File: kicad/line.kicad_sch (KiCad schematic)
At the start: 40 parts, among them J11 AudioJack3, J2 AudioJack3, U12 NE5532, U13 NE5532, U14 NE5532, U15 NE5532

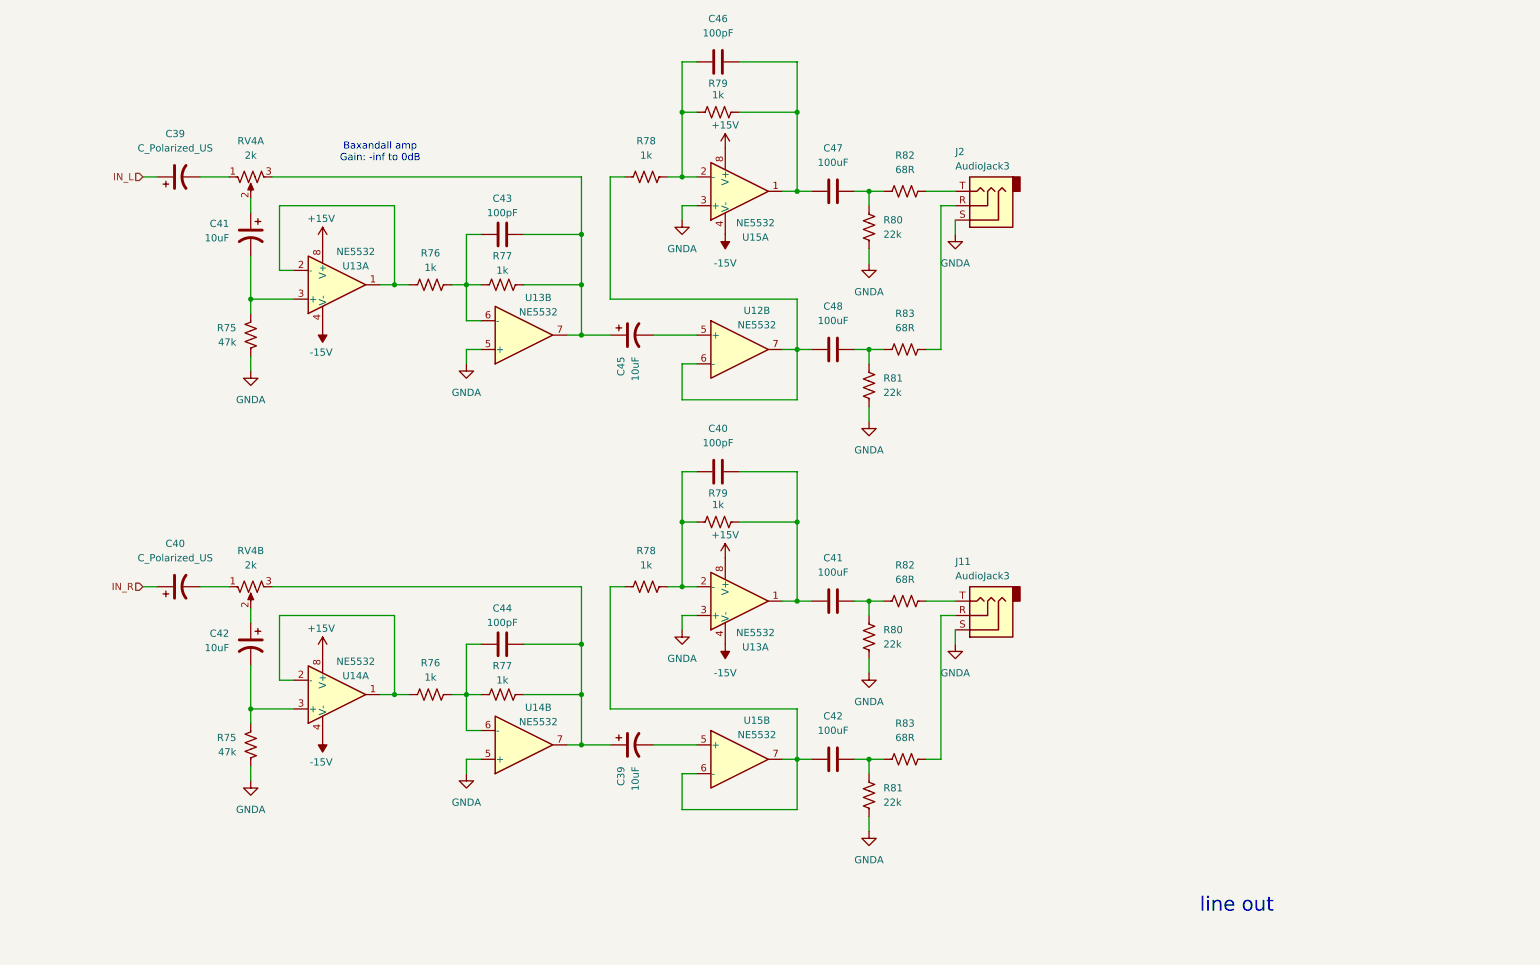
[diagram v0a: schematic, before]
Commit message: tac5212 initial architecture
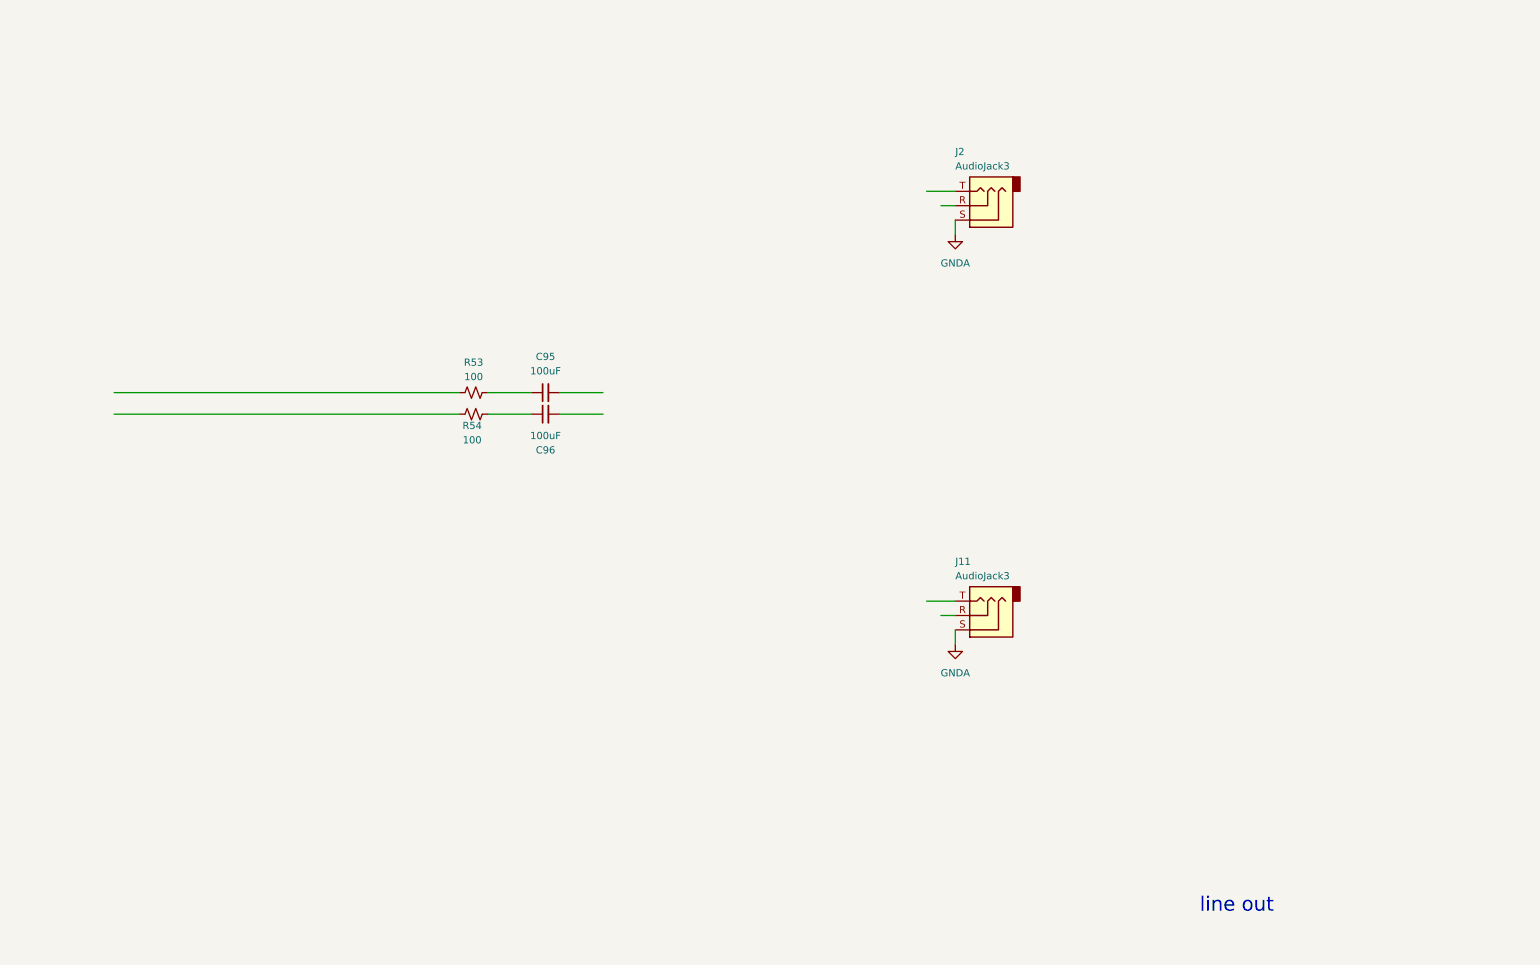
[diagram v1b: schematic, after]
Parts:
- removed C39, C40: C_Polarized_US, symbol Device:C_Polarized_US
- removed C39, C41, C42, C45: 10uF, symbol Device:C_Polarized_US
- removed C40, C43, C44, C46: 100pF, symbol Device:C
- removed C41, C42, C47, C48: 100uF, symbol Device:C
- removed R75 (x2): 47k, symbol Device:R_US
- removed R76 (x2), R77 (x2), R78 (x2), R79 (x2): 1k, symbol Device:R_US
- removed R80 (x2), R81 (x2): 22k, symbol Device:R_US
- removed R82 (x2), R83 (x2): 68R, symbol Device:R_US
- removed RV4: 2k, symbol openmic:R_Potentiometer_US_Dual
- removed U12, U13, U14, U15: NE5532, symbol Amplifier_Operational:NE5532
- added C95, C96: 100uF, symbol Device:C_Small
- added R53, R54: 100, symbol Device:R_Small_US
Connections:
- new net: C95.1, R53.2
- new net: C96.1, R54.2
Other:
- note removed: "Baxandall amp Gain: -inf to 0dB"

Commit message: line out
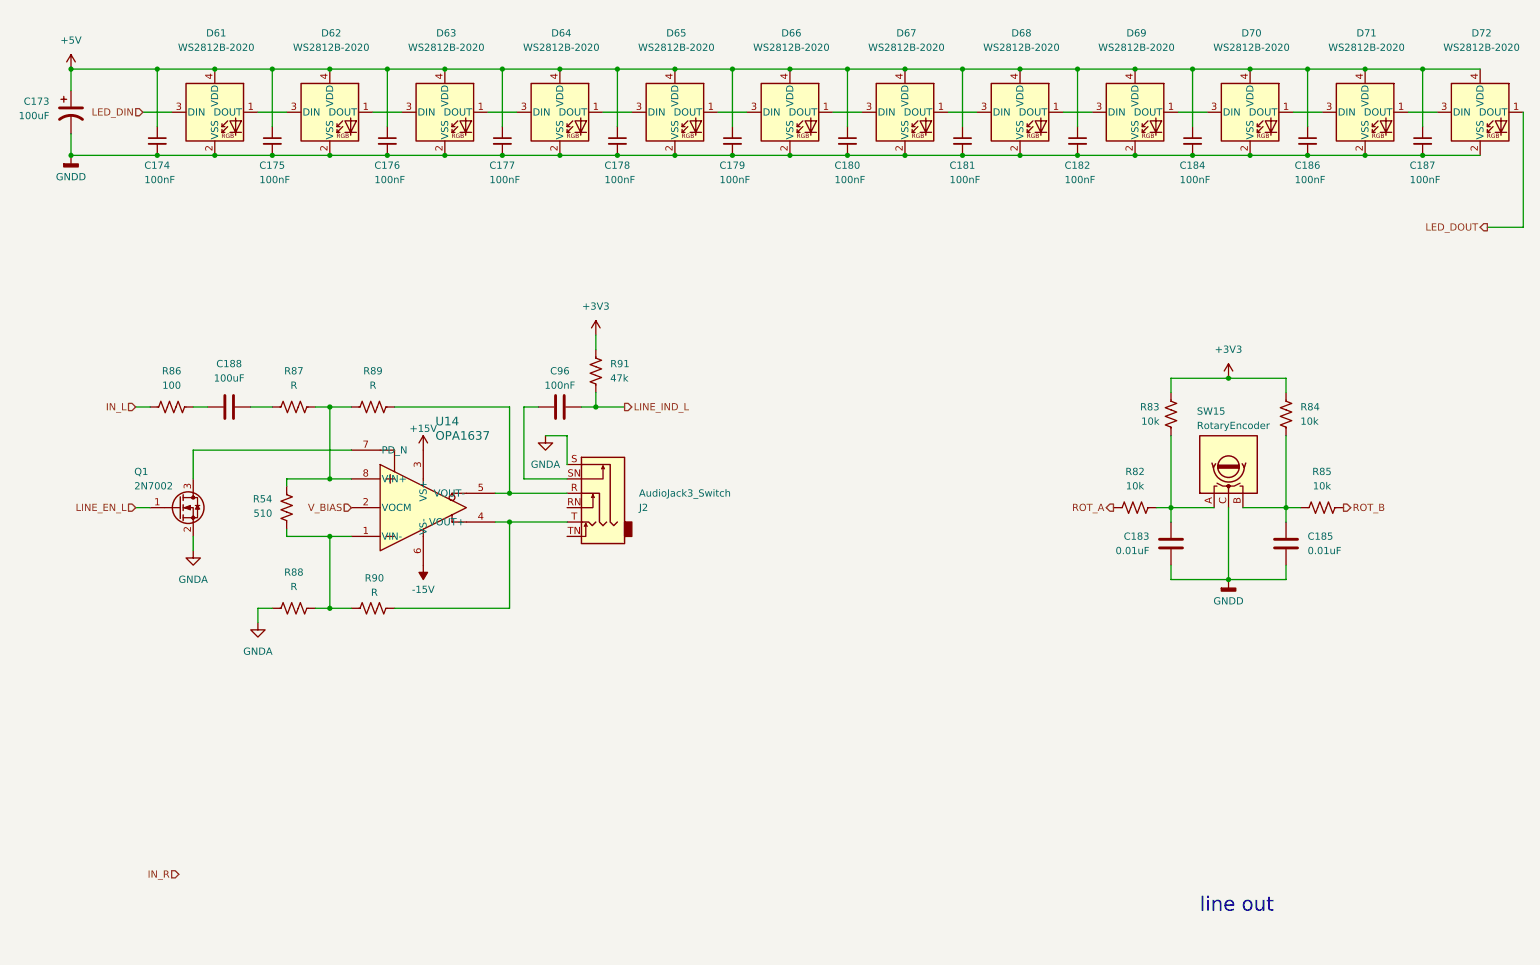
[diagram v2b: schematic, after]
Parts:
- removed C95, C96: 100uF, symbol Device:C_Small
- removed J11, J2: AudioJack3, symbol Connector_Audio:AudioJack3
- removed R53, R54: 100, symbol Device:R_Small_US
- added C173: 100uF, symbol Device:C_Polarized_US
- added C174, C175, C176, C177, C178, C179, C180, C181, C182, C184, C186, C187: 100nF, symbol Device:C_Small
- added C183, C185: 0.01uF, symbol Device:C
- added C188: 100uF, symbol Device:C
- added C96: 100nF, symbol Device:C
- added D61, D62, D63, D64, D65, D66, D67, D68, D69, D70, D71, D72: WS2812B-2020, LED_SMD:LED_WS2812B-2020_PLCC4_2.0x2.0mm, symbol LED:WS2812B-2020
- added J2: AudioJack3_Switch, symbol Connector_Audio:AudioJack3_Switch
- added Q1: 2N7002, Package_TO_SOT_SMD:SOT-23, symbol Transistor_FET:2N7002
- added R54: 510, symbol Device:R_US
- added R82, R83, R84, R85: 10k, symbol Device:R_US
- added R86: 100, symbol Device:R_US
- added R87, R88, R89, R90: R, symbol Device:R_US
- added R91: 47k, symbol Device:R_US
- added SW15: RotaryEncoder, symbol Device:RotaryEncoder
- added U14: OPA1637, DGK0008A_N, symbol openmic:OPA1637
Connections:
- net GNDA: now also J2.S, Q1.2 (S), R88.1
- new net: C96.1, J2.SN
- new net: D69.1 (DOUT), D70.3 (DIN)
- new net: D68.1 (DOUT), D69.3 (DIN)
- new net: D67.1 (DOUT), D68.3 (DIN)
- new net: D66.1 (DOUT), D67.3 (DIN)
- new net: J2.T, R90.1, U14.4 (VOUT+)
- new net: R54.1, R88.2, R90.2, U14.1 (VIN-)
- new net: D71.1 (DOUT), D72.3 (DIN)
- new net: D70.1 (DOUT), D71.3 (DIN)
- new net: C183.1, R82.2, R83.1, SW15.A
- new net: C185.1, R84.2, R85.1, SW15.B
- new net: R54.2, R87.2, R89.1, U14.8 (VIN+)
- new net: J2.R, R89.2, U14.5 (VOUT-)
- new net: D65.1 (DOUT), D66.3 (DIN)
- new net: D64.1 (DOUT), D65.3 (DIN)
- new net: Q1.3 (D), U14.7 (PD_N)
- new net: D61.1 (DOUT), D62.3 (DIN)
- new net: D63.1 (DOUT), D64.3 (DIN)
- new net: D62.1 (DOUT), D63.3 (DIN)
- new net: C188.1, R86.2
- new net: C188.2, R87.1
- new net +15V: U14.3 (VS+)
- new net +3V3: R83.2, R84.1, R91.1
- new net +5V: C173.1, C174.1, C175.1, C176.1, C177.1, C178.1, C179.1, C180.1, C181.1, C182.1, C184.1, C186.1, C187.1, D61.4 (VDD), D62.4 (VDD), D63.4 (VDD), D64.4 (VDD), D65.4 (VDD), D66.4 (VDD), D67.4 (VDD), D68.4 (VDD), D69.4 (VDD), D70.4 (VDD), D71.4 (VDD), D72.4 (VDD)
- new net -15V: U14.6 (VS-)
- new net GNDD: C173.2, C174.2, C175.2, C176.2, C177.2, C178.2, C179.2, C180.2, C181.2, C182.2, C183.2, C184.2, C185.2, C186.2, C187.2, D61.2 (VSS), D62.2 (VSS), D63.2 (VSS), D64.2 (VSS), D65.2 (VSS), D66.2 (VSS), D67.2 (VSS), D68.2 (VSS), D69.2 (VSS), D70.2 (VSS), D71.2 (VSS), D72.2 (VSS), SW15.C
- new net IN_L: R86.1
- new net LED_DIN: D61.3 (DIN)
- new net LED_DOUT: D72.1 (DOUT)
- new net LINE_EN_L: Q1.1 (G)
- new net LINE_IND_L: C96.2, R91.2
- new net ROT_A: R82.1
- new net ROT_B: R85.2
- new net V_BIAS: U14.2 (VOCM)

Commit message: line out
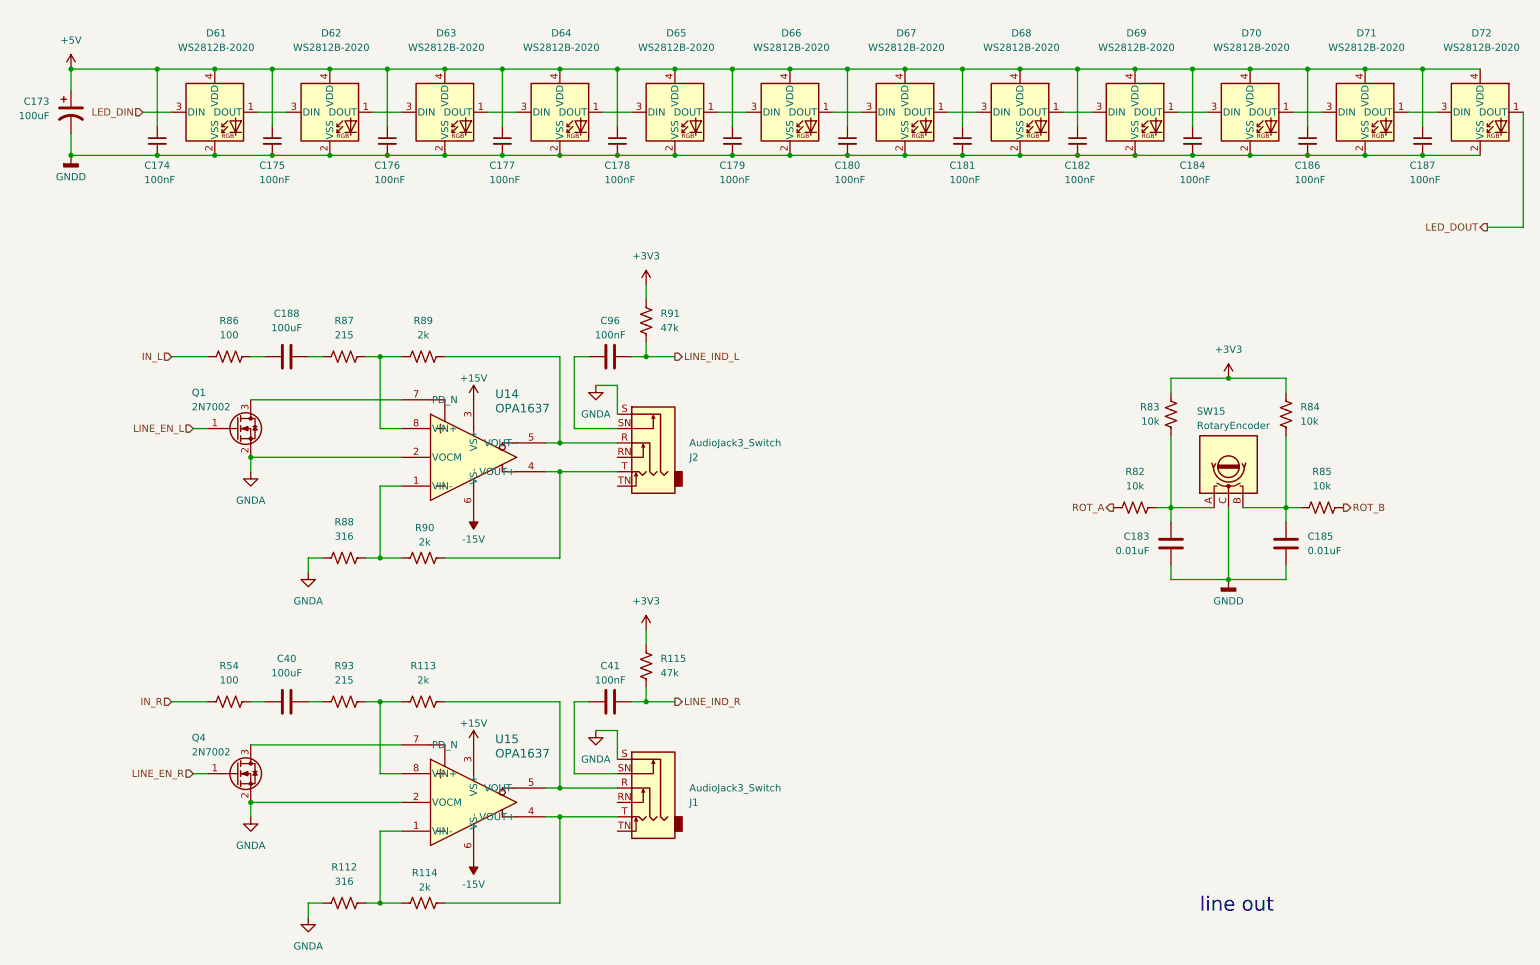
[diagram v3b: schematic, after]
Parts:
- added C40: 100uF, symbol Device:C
- added C41: 100nF, symbol Device:C
- added J1: AudioJack3_Switch, symbol Connector_Audio:AudioJack3_Switch
- added Q4: 2N7002, Package_TO_SOT_SMD:SOT-23, symbol Transistor_FET:2N7002
- added R112: 316, symbol Device:R_US
- added R113, R114: 2k, symbol Device:R_US
- added R115: 47k, symbol Device:R_US
- added R93: 215, symbol Device:R_US
- added U15: OPA1637, DGK0008A_N, symbol openmic:OPA1637
- R54: value 510 -> 100
- R87: value R -> 215
- R88: value R -> 316
- R89, R90: value R -> 2k
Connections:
- net V_BIAS is gone; now on net GNDA: U14.2 (VOCM)
- net +15V: now also U15.3 (VS+)
- net +3V3: now also R115.1
- net -15V: now also U15.6 (VS-)
- net GNDA: now also J1.S, Q4.2 (S), R112.1, U15.2 (VOCM)
- net IN_R: now also R54.1
- net at R88.2, R90.2, U14.1 (VIN-): no longer R54.1
- net at R87.2, R89.1, U14.8 (VIN+): no longer R54.2
- new net: J1.R, R113.2, U15.5 (VOUT-)
- new net: C41.1, J1.SN
- new net: J1.T, R114.1, U15.4 (VOUT+)
- new net: R112.2, R114.2, U15.1 (VIN-)
- new net: Q4.3 (D), U15.7 (PD_N)
- new net: R113.1, R93.2, U15.8 (VIN+)
- new net: C40.1, R54.2
- new net: C40.2, R93.1
- new net LINE_EN_R: Q4.1 (G)
- new net LINE_IND_R: C41.2, R115.2
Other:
- moved on the sheet: C188, C96, J2, Q1, R86, R87, R88, R89, R90, R91, U14
